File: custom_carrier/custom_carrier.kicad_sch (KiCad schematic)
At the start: 2 parts, among them J1 ERF5-040-05.0-X-DV, J2 ERF5-040-05.0-X-DV

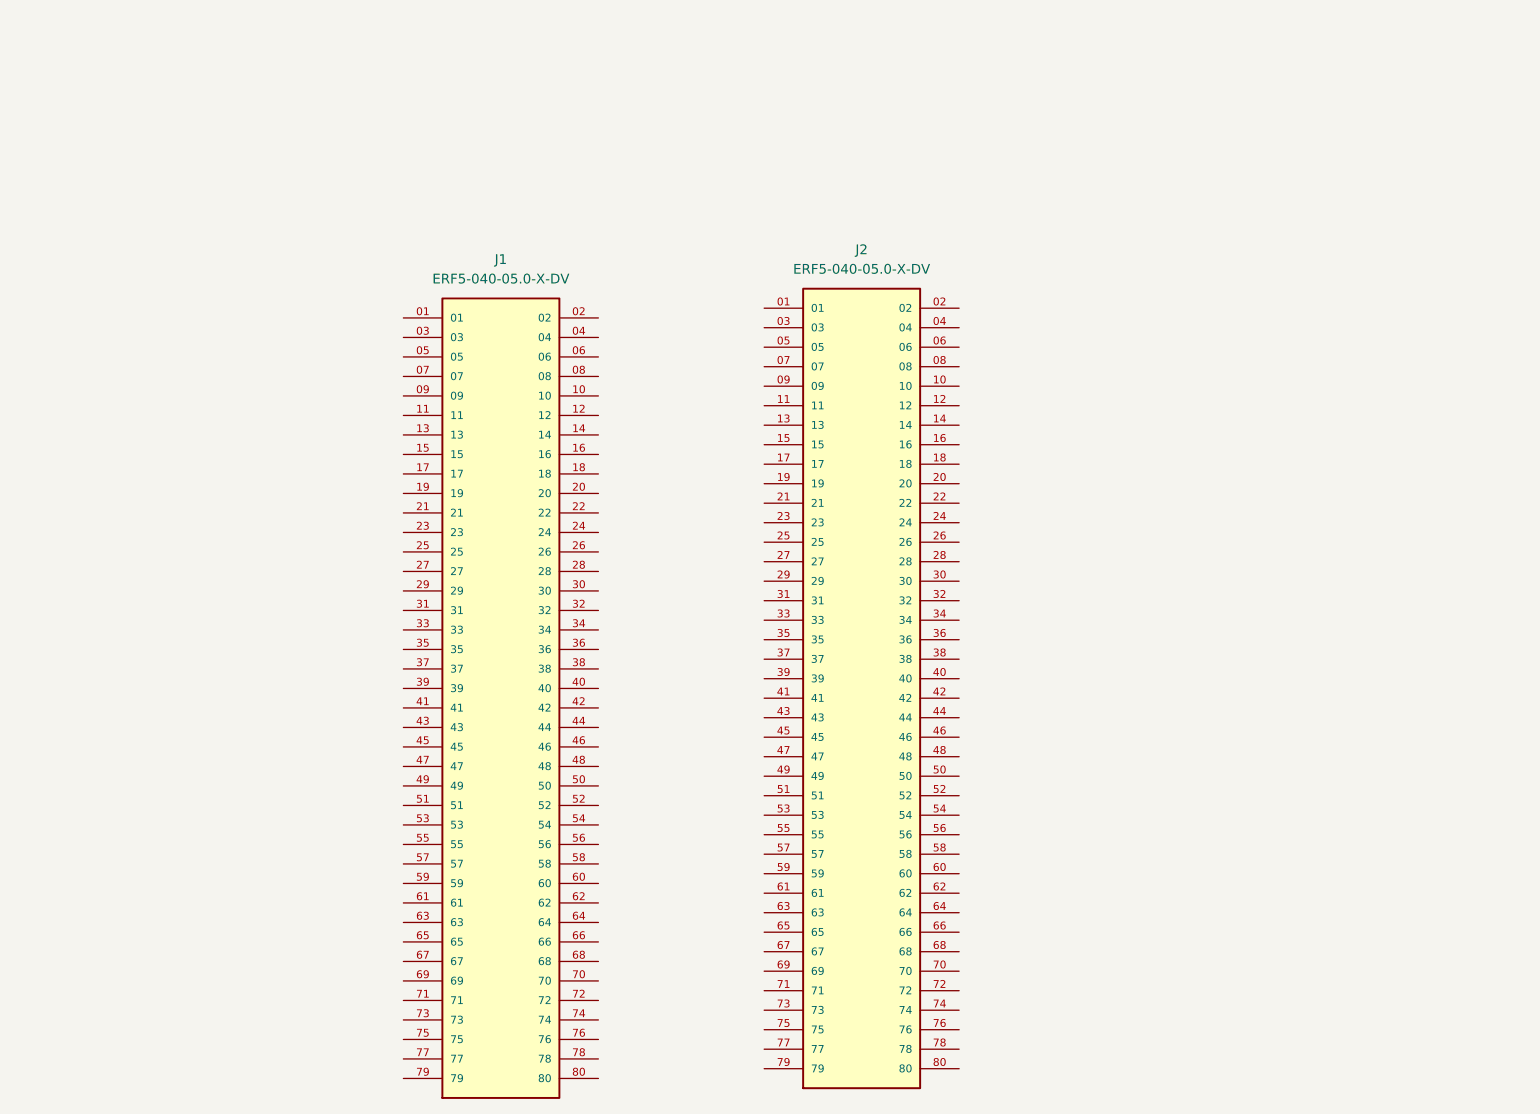
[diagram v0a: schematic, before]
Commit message: working on custom carrier in V7
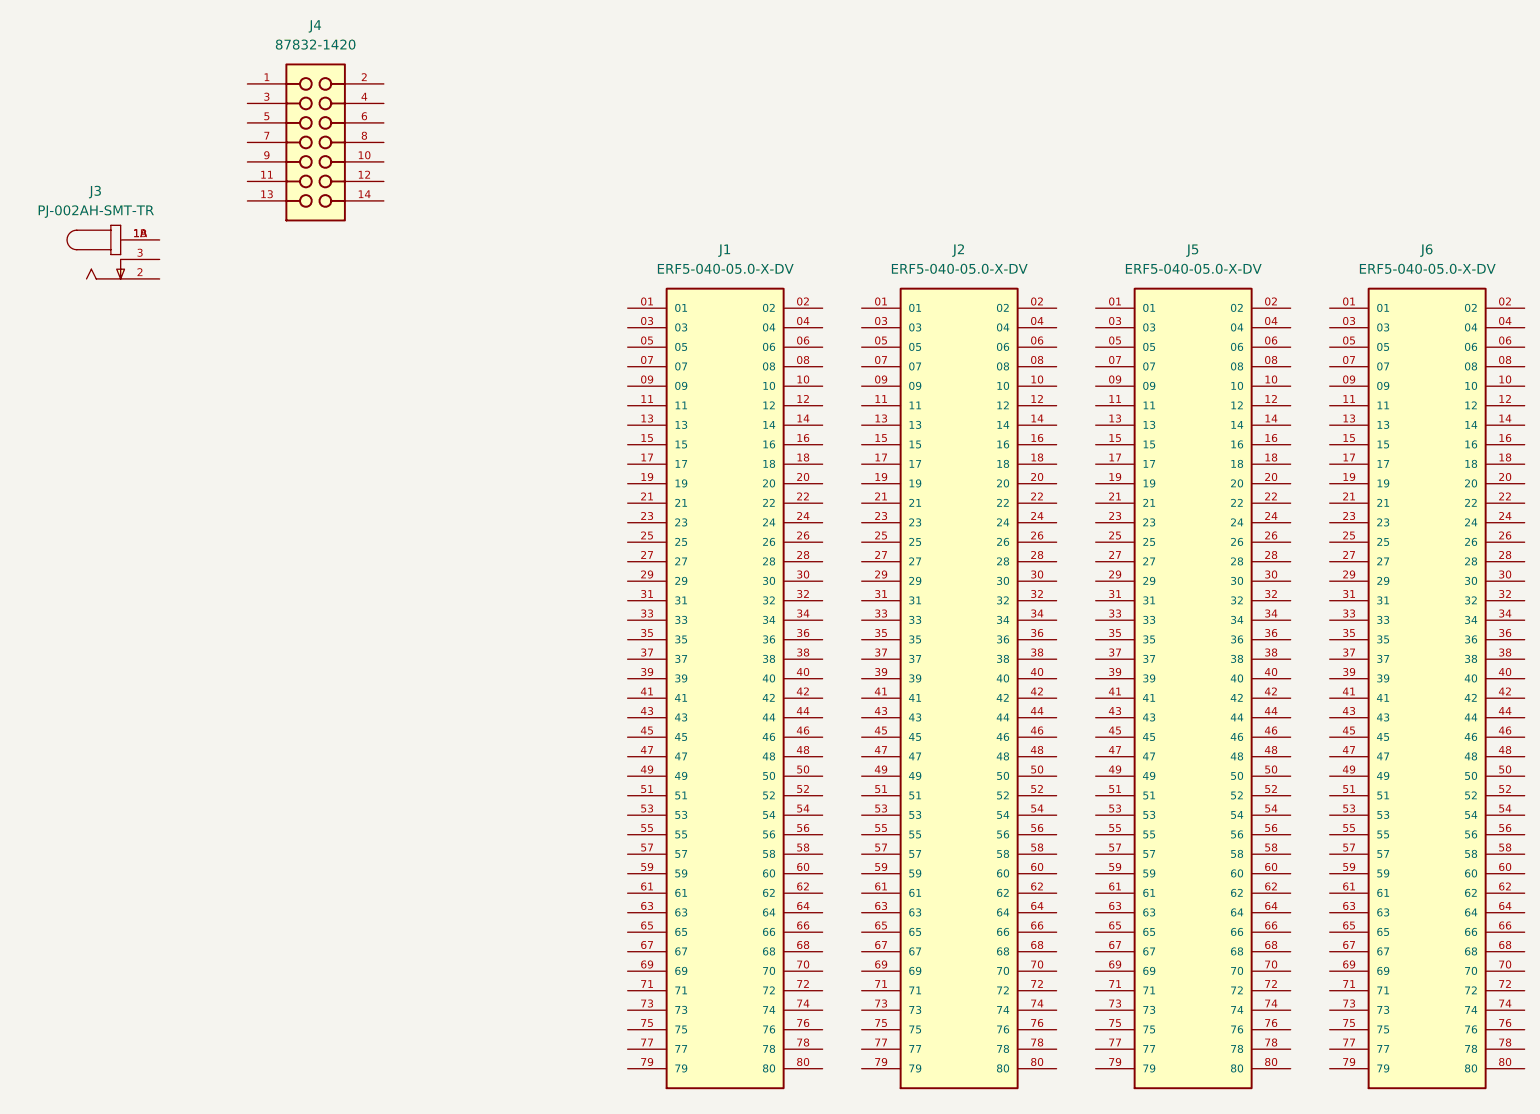
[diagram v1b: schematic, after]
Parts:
- added J3: PJ-002AH-SMT-TR, pedrolib:CUI_PJ-002AH-SMT-TR, symbol pedrolib:PJ-002AH-SMT-TR
- added J4: 87832-1420, pedrolib:MOLEX_87832-1420, symbol pedrolib:87832-1420
- added J5, J6: ERF5-040-05.0-X-DV, pedrolib:SAMTEC_ERF5-040-05.0-X-DV, symbol pedrolib:ERF5-040-05.0-X-DV
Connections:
- new net: J3.1A, J3.1B
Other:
- moved on the sheet: J1, J2
